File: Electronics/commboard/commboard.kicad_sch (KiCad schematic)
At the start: 73 parts, among them J101 USB_B, J102 PowerConn, J103 LED CONN, J104 ReservedIO_0, J105 ReservedIO_1, J106 STLINK, J107 ProximitySensorConnector, J108 RS232_Out, J109 24V Power In, J110 RS485_Out_1, J111 RS485_Out_1, Q101 BC847, Q102 BSS83P, SW101 SW_Push, U101 STM32F070CBTx, U102 LM2576HVS-3.3, U103 M24C08, U104 MAX3221, U105 SP3485EN, U106 SP3485EN, Y101 8MHz

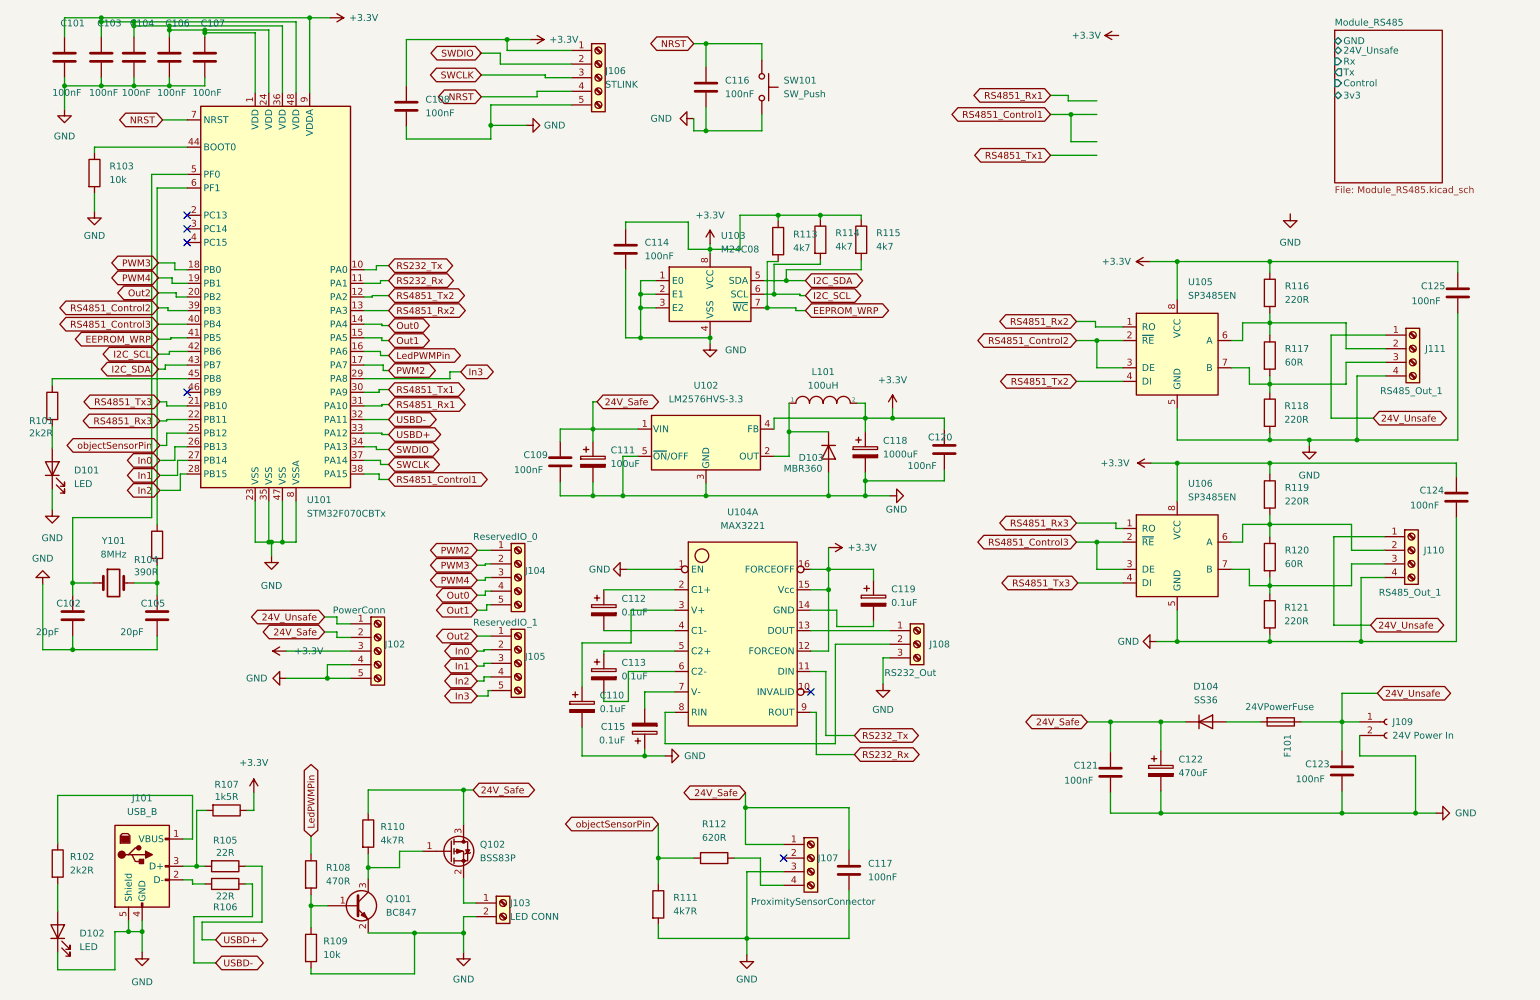
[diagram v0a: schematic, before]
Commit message: completed pcb design
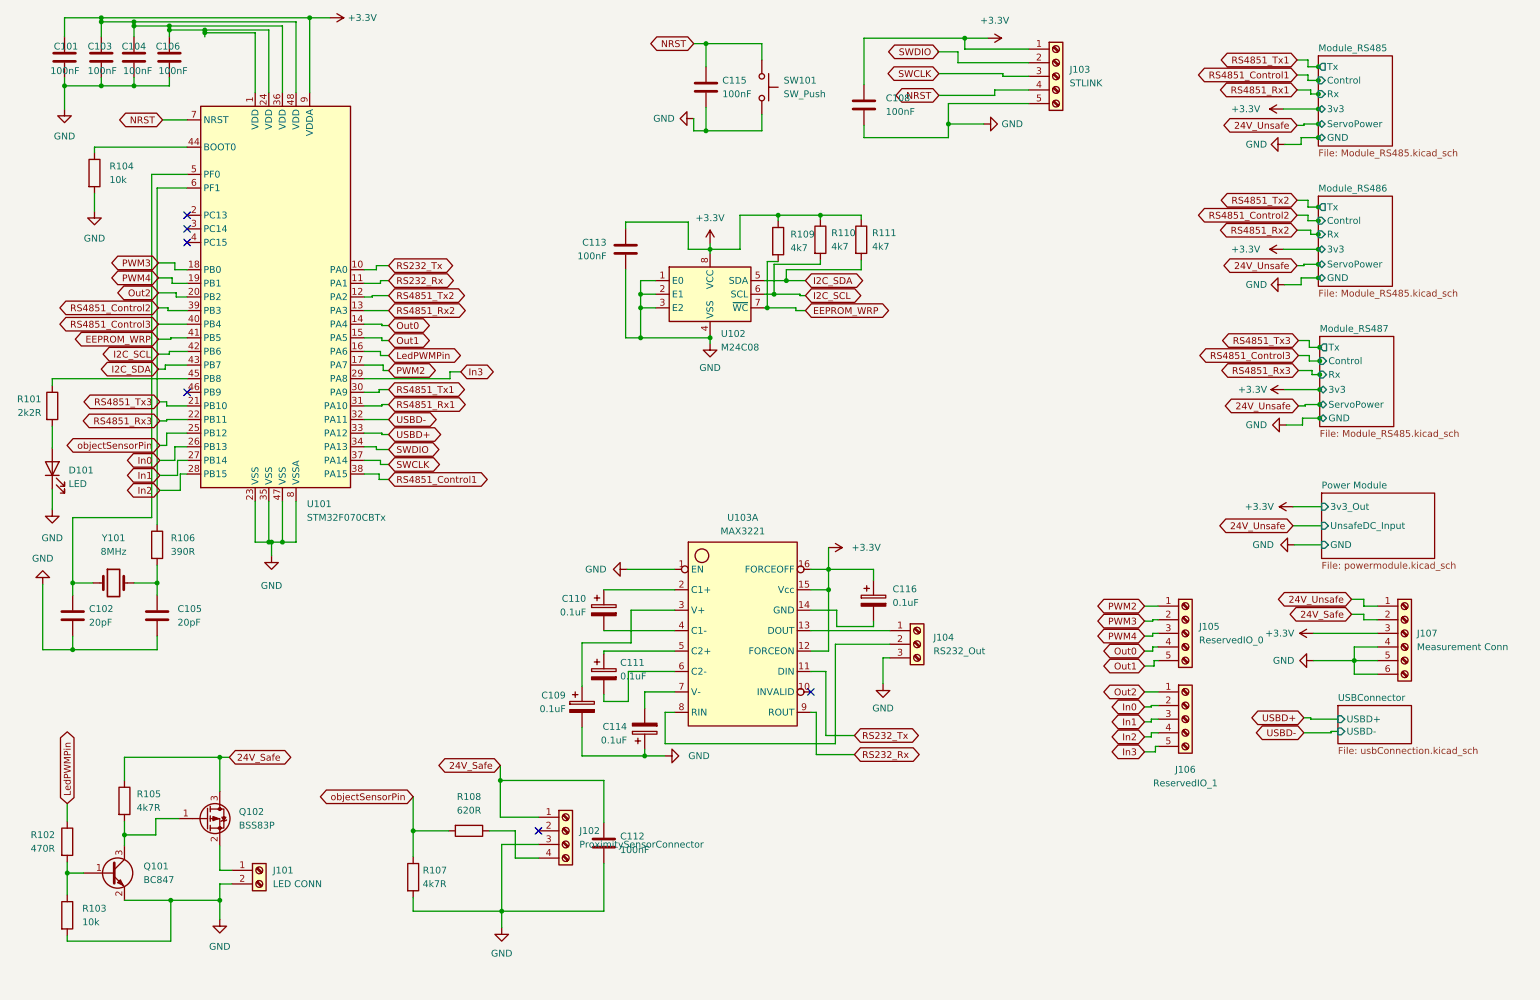
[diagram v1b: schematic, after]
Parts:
- removed C107, C109, C121, C123: 100nF, Capacitor_THT:C_Rect_L7.0mm_W2.0mm_P5.00mm, symbol Device:C
- removed C111: 100uF, Capacitor_THT:CP_Radial_D22.0mm_P10.00mm_SnapIn, symbol Device:C_Polarized
- removed C118: 1000uF, Capacitor_THT:CP_Radial_D22.0mm_P10.00mm_SnapIn, symbol Device:C_Polarized
- removed C120, C124, C125: 100nF, Capacitor_SMD:C_0805_2012Metric, symbol Device:C
- removed C122: 470uF, Capacitor_THT:CP_Radial_D22.0mm_P10.00mm_SnapIn, symbol Device:C_Polarized
- removed D102: LED, Diode_SMD:D_0805_2012Metric, symbol Device:LED
- removed D103: MBR360, Diode_SMD:D_SMA, symbol Diode:1N4148
- removed D104: SS36, Diode_SMD:D_SMA, symbol Diode:1N4148
- removed F101: 24VPowerFuse, Resistor_SMD:R_1206_3216Metric, symbol Device:Fuse
- removed J101: USB_B, Connector_USB:USB_B_OST_USB-B1HSxx_Horizontal, symbol Connector:USB_B
- removed J109: 24V Power In, Connector_PinSocket_2.00mm:PinSocket_1x02_P2.00mm_Vertical, symbol Connector:Conn_01x02_Female
- removed J110, J111: RS485_Out_1, symbol Connector:Screw_Terminal_01x04
- removed L101: 100uH, Inductor_SMD:L_12x12mm_H8mm, symbol pspice:INDUCTOR
- removed R102: 2k2R, Resistor_SMD:R_0805_2012Metric, symbol Device:R
- removed R105, R106: 22R, Resistor_SMD:R_0805_2012Metric, symbol Device:R
- removed R107: 1k5R, Resistor_SMD:R_0805_2012Metric, symbol Device:R
- removed R116, R118, R119, R121: 220R, Resistor_SMD:R_0805_2012Metric, symbol Device:R
- removed R117, R120: 60R, Resistor_SMD:R_0805_2012Metric, symbol Device:R
- removed U102: LM2576HVS-3.3, Package_TO_SOT_SMD:TO-263-5_TabPin3, symbol Regulator_Switching:LM2576HVS-3.3
- removed U105, U106: SP3485EN, Package_SO:SOIC-8_3.9x4.9mm_P1.27mm, symbol Interface_UART:SP3485EN
- C101, C103, C104, C106: footprint Capacitor_THT:C_Rect_L7.0mm_W2.0mm_P5.00mm -> Capacitor_SMD:C_0805_2012Metric
- C109: renamed from C110; footprint (none) -> Capacitor_THT:CP_Radial_D5.0mm_P2.50mm
- C110: renamed from C112; footprint (none) -> Capacitor_THT:CP_Radial_D5.0mm_P2.50mm
- C111: renamed from C113; footprint (none) -> Capacitor_THT:CP_Radial_D5.0mm_P2.50mm
- C114: renamed from C115; footprint (none) -> Capacitor_THT:CP_Radial_D5.0mm_P2.50mm
- C116: renamed from C119; footprint (none) -> Capacitor_THT:CP_Radial_D5.0mm_P2.50mm
- J101: renamed from J103; footprint Connector_PinSocket_2.00mm:PinSocket_1x02_P2.00mm_Vertical -> Connector_PinHeader_2.54mm:PinHeader_1x02_P2.54mm_Vertical
- J102: renamed from J107; footprint Connector_PinSocket_2.54mm:PinSocket_1x04_P2.54mm_Vertical -> Connector_PinHeader_2.54mm:PinHeader_1x04_P2.54mm_Vertical
- J103: renamed from J106; footprint Connector_PinSocket_1.00mm:PinSocket_1x05_P1.00mm_Vertical -> Connector_PinHeader_2.54mm:PinHeader_1x05_P2.54mm_Vertical
- J104: renamed from J108; footprint (none) -> Connector_PinHeader_2.54mm:PinHeader_1x03_P2.54mm_Vertical
- J105: renamed from J104; footprint Connector_PinSocket_1.00mm:PinSocket_1x05_P1.00mm_Vertical -> Connector_PinHeader_2.54mm:PinHeader_1x05_P2.54mm_Vertical
- J106: renamed from J105; footprint Connector_PinSocket_1.00mm:PinSocket_1x05_P1.00mm_Vertical -> Connector_PinHeader_2.54mm:PinHeader_1x05_P2.54mm_Vertical
- J107: renamed from J102; value PowerConn -> Measurement Conn; footprint Connector_PinSocket_1.00mm:PinSocket_1x05_P1.00mm_Vertical -> Connector_PinHeader_2.54mm:PinHeader_1x06_P2.54mm_Vertical; symbol Connector:Screw_Terminal_01x05 -> Connector:Screw_Terminal_01x06
- SW101: footprint (none) -> Button_Switch_SMD:SW_Push_1P1T_NO_CK_KSC7xxJ
- renumbered C117 to C112, C114 to C113, C116 to C115, R108 to R102, R109 to R103, R103 to R104, R110 to R105, R104 to R106, R111 to R107, R112 to R108, R113 to R109, R114 to R110, R115 to R111, U103 to U102, U104 to U103
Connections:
- net GND: now also J107.6 (Pin_6)
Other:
- added sheet Module_RS486 (Module_RS485.kicad_sch)
- added sheet Module_RS487 (Module_RS485.kicad_sch)
- added sheet Power Module (powermodule.kicad_sch)
- added sheet USBConnector (usbConnection.kicad_sch)
- sheet Module_RS485 ports: added ServoPower; removed 24V_Unsafe
- moved on the sheet: C108, C112, J101, J102, J103, J105, J106, Q101, Q102, R102, R103, R105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
